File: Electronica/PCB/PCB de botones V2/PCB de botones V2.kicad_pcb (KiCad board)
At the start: 2 copper layers, 56.1 x 32.5 mm, 11 parts, among them J1 IDC Placa Botones, SW1 SW_Push, SW2 SW_Push

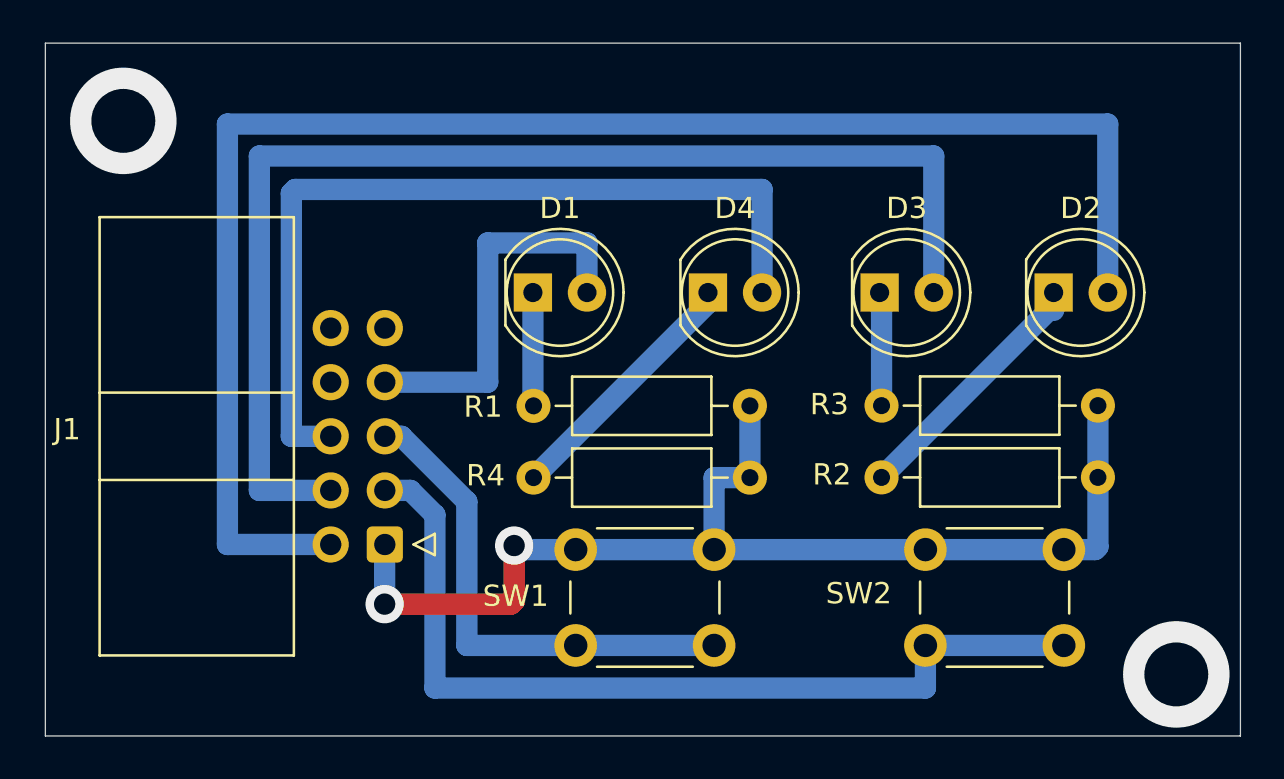
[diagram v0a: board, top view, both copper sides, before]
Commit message: prueba de botones, contador binario
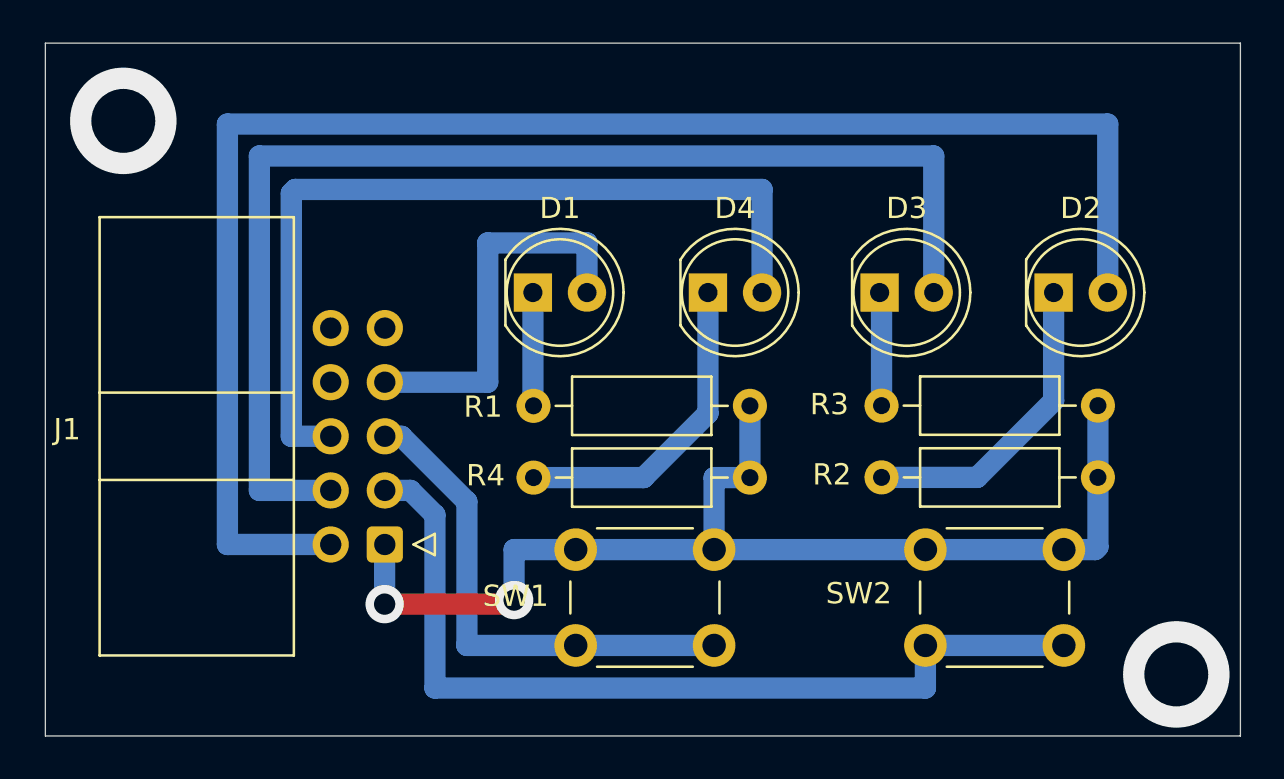
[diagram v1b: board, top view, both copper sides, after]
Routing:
- net Net-(D4-K): track 12.1 -> 15.1 mm
- net Net-(D2-K): track 12.9 -> 14.7 mm
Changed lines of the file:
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@@
 		)
 		(fp_text user "${REFERENCE}"
-			(at 8.83 5.08 270)
+			(at 8.83 5.08 -90)
 			(layer "F.Fab")
 			(effects
@@
 	)
 	(segment
+		(start 139.36 85.96)
+		(end 139.38 85.98)
+		(width 1)
+		(layer "F.Cu")
+		(net 3)
+	)
+	(segment
 		(start 139.38 85.98)
 		(end 139.21 86.15)
-		(width 1)
-		(layer "F.Cu")
-		(net 3)
-	)
-	(segment
-		(start 139.36 83.4)
-		(end 139.36 85.96)
-		(width 1)
-		(layer "F.Cu")
-		(net 3)
-	)
-	(segment
-		(start 139.36 85.96)
-		(end 139.38 85.98)
 		(width 1)
 		(layer "F.Cu")
@@
 	)
 	(via
-		(at 139.36 83.4)
+		(at 139.36 85.96)
 		(size 1.8)
 		(drill 1)
@@
 	)
 	(segment
-		(start 142.25 83.59)
-		(end 139.55 83.59)
-		(width 1)
-		(layer "B.Cu")
-		(net 3)
-	)
-	(segment
 		(start 165.17 83.59)
 		(end 158.67 83.59)
@@
 	)
 	(segment
+		(start 139.36 85.96)
+		(end 139.36 83.59)
+		(width 1)
+		(layer "B.Cu")
+		(net 3)
+	)
+	(segment
 		(start 148.75 83.59)
 		(end 148.75 80.21)
@@
 	)
 	(segment
+		(start 139.36 83.59)
+		(end 142.25 83.59)
+		(width 1)
+		(layer "B.Cu")
+		(net 3)
+	)
+	(segment
 		(start 150.43 76.84)
 		(end 150.43 80.21)
@@
 	)
 	(segment
-		(start 139.55 83.59)
-		(end 139.36 83.4)
-		(width 1)
-		(layer "B.Cu")
-		(net 3)
-	)
-	(segment
 		(start 142.78 69.19)
 		(end 138.12 69.19)
@@
 	)
 	(segment
-		(start 164.69 72.36)
-		(end 164.69 71.52)
+		(start 164.69 76.61)
+		(end 161.1 80.2)
 		(width 1)
 		(layer "B.Cu")
@@
 	)
 	(segment
-		(start 164.69 72.12)
+		(start 164.69 71.52)
+		(end 164.69 76.61)
+		(width 1)
+		(layer "B.Cu")
+		(net 6)
+	)
+	(segment
+		(start 161.1 80.2)
 		(end 156.61 80.2)
-		(width 1)
-		(layer "B.Cu")
-		(net 6)
-	)
-	(segment
-		(start 164.69 71.52)
-		(end 164.69 72.12)
 		(width 1)
 		(layer "B.Cu")
@@
 	)
 	(segment
-		(start 148.46 72.02)
+		(start 145.44 80.21)
+		(end 148.46 77.19)
+		(width 1)
+		(layer "B.Cu")
+		(net 8)
+	)
+	(segment
+		(start 140.27 80.21)
+		(end 145.44 80.21)
+		(width 1)
+		(layer "B.Cu")
+		(net 8)
+	)
+	(segment
+		(start 148.46 77.19)
 		(end 148.46 71.52)
 		(width 1)
 		(layer "B.Cu")
-		(net 8)
-	)
-	(segment
-		(start 140.27 80.21)
-		(end 148.46 72.02)
-		(width 1)
-		(layer "B.Cu")
